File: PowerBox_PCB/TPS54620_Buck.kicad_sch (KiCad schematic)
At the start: 17 parts

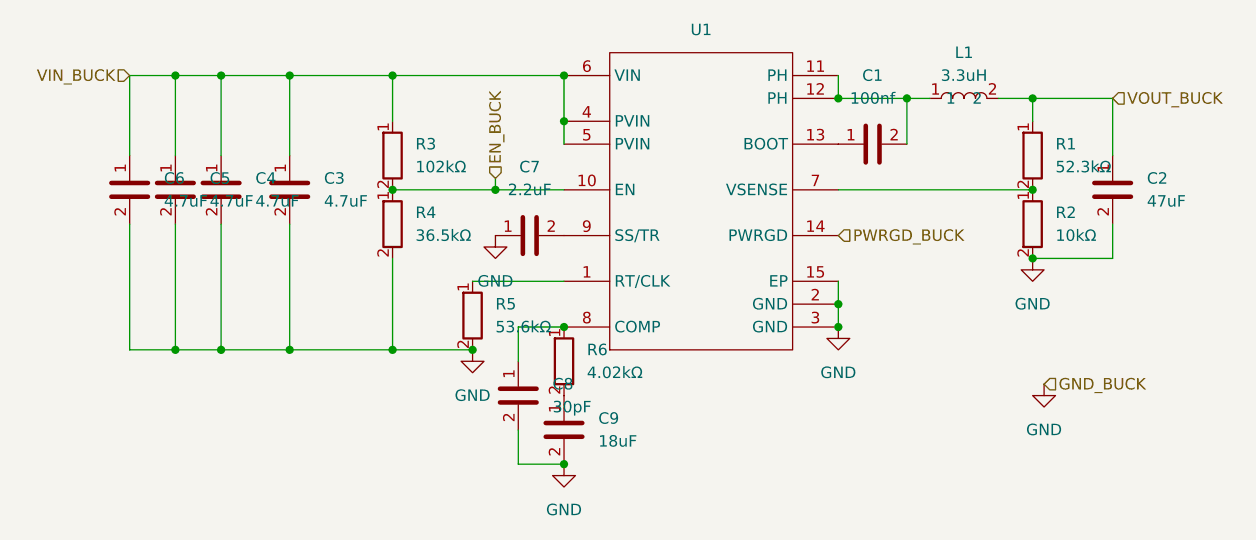
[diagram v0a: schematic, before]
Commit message: .
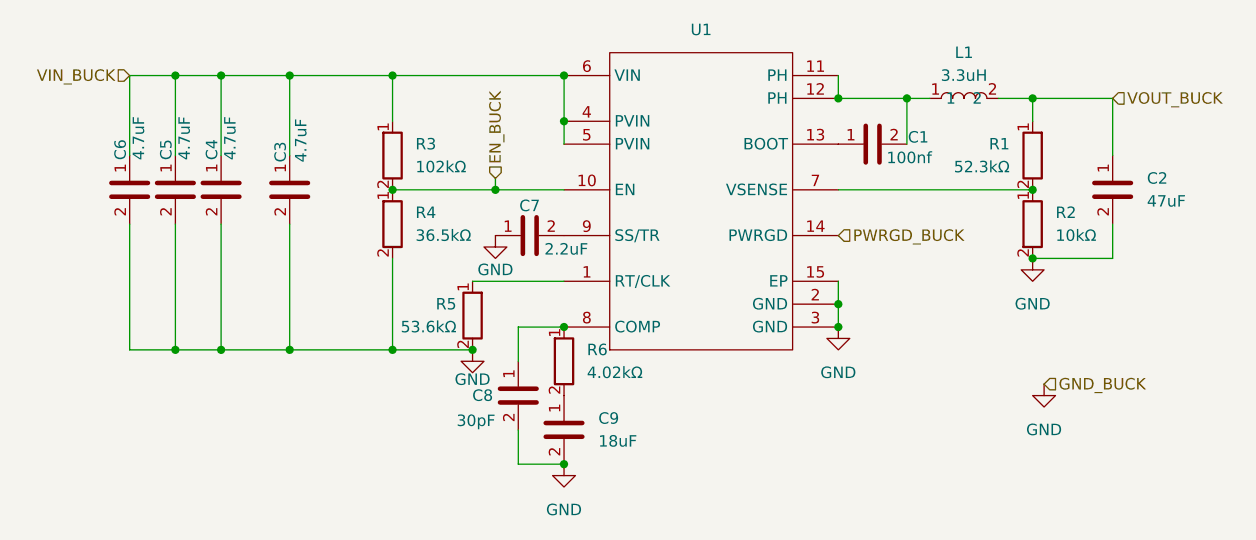
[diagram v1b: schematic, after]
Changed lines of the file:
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@@
 		(lib_id "Buck_TPS54620:30pF_Cap_0805")
 		(at 119.38 115.57 0)
-		(unit 1)
-		(body_style 1)
-		(exclude_from_sim no)
-		(in_bom yes)
-		(on_board yes)
-		(in_pos_files yes)
-		(dnp no)
-		(fields_autoplaced yes)
+		(mirror y)
+		(unit 1)
+		(body_style 1)
+		(exclude_from_sim no)
+		(in_bom yes)
+		(on_board yes)
+		(in_pos_files yes)
+		(dnp no)
 		(property "Reference" "C8"
-			(at 123.19 114.2999 0)
+			(at 116.586 115.57 0)
 			(show_name no)
 			(do_not_autoplace no)
@@
 		)
 		(property "Value" "30pF"
-			(at 123.19 116.8399 0)
+			(at 116.84 118.364 0)
 			(show_name no)
 			(do_not_autoplace no)
@@
 		(lib_id "Buck_TPS54620:53.6kΩ_Res_0805")
 		(at 114.3 106.68 0)
-		(unit 1)
-		(body_style 1)
-		(exclude_from_sim no)
-		(in_bom yes)
-		(on_board yes)
-		(in_pos_files yes)
-		(dnp no)
-		(fields_autoplaced yes)
+		(mirror y)
+		(unit 1)
+		(body_style 1)
+		(exclude_from_sim no)
+		(in_bom yes)
+		(on_board yes)
+		(in_pos_files yes)
+		(dnp no)
 		(property "Reference" "R5"
-			(at 116.84 105.4099 0)
+			(at 112.522 105.41 0)
 			(show_name no)
 			(do_not_autoplace no)
@@
 		)
 		(property "Value" "53.6kΩ"
-			(at 116.84 107.9499 0)
+			(at 112.522 107.95 0)
 			(show_name no)
 			(do_not_autoplace no)
@@
 		(in_pos_files yes)
 		(dnp no)
-		(fields_autoplaced yes)
 		(property "Reference" "C7"
-			(at 120.65 90.17 90)
+			(at 120.65 94.488 90)
 			(show_name no)
 			(do_not_autoplace no)
@@
 		)
 		(property "Value" "2.2uF"
-			(at 120.65 92.71 90)
+			(at 124.714 99.314 90)
 			(show_name no)
 			(do_not_autoplace no)
@@
 		(in_pos_files yes)
 		(dnp no)
-		(fields_autoplaced yes)
 		(property "Reference" "C5"
-			(at 85.09 91.4399 0)
+			(at 80.264 89.408 90)
 			(show_name no)
 			(do_not_autoplace no)
@@
 		)
 		(property "Value" "4.7uF"
-			(at 85.09 93.9799 0)
+			(at 82.296 89.408 90)
 			(show_name no)
 			(do_not_autoplace no)
@@
 		(in_pos_files yes)
 		(dnp no)
-		(fields_autoplaced yes)
 		(property "Reference" "C6"
-			(at 80.01 91.4399 0)
+			(at 75.184 89.408 90)
 			(show_name no)
 			(do_not_autoplace no)
@@
 		)
 		(property "Value" "4.7uF"
-			(at 80.01 93.9799 0)
+			(at 77.216 89.408 90)
 			(show_name no)
 			(do_not_autoplace no)
@@
 		(in_pos_files yes)
 		(dnp no)
-		(fields_autoplaced yes)
 		(property "Reference" "C4"
-			(at 90.17 91.4399 0)
+			(at 85.344 89.408 90)
 			(show_name no)
 			(do_not_autoplace no)
@@
 		)
 		(property "Value" "4.7uF"
-			(at 90.17 93.9799 0)
+			(at 87.376 89.408 90)
 			(show_name no)
 			(do_not_autoplace no)
@@
 		(in_pos_files yes)
 		(dnp no)
-		(fields_autoplaced yes)
 		(property "Reference" "C3"
-			(at 97.79 91.4399 0)
+			(at 92.964 89.662 90)
 			(show_name no)
 			(do_not_autoplace no)
@@
 		)
 		(property "Value" "4.7uF"
-			(at 97.79 93.9799 0)
+			(at 95.25 89.662 90)
 			(show_name no)
 			(do_not_autoplace no)
@@
 		(in_pos_files yes)
 		(dnp no)
-		(fields_autoplaced yes)
 		(property "Reference" "#PWR04"
 			(at 116.84 104.14 0)
@@
 		)
 		(property "Value" "GND"
-			(at 116.84 102.87 0)
+			(at 116.84 101.6 0)
 			(show_name no)
 			(do_not_autoplace no)
@@
 		(in_pos_files yes)
 		(dnp no)
-		(fields_autoplaced yes)
 		(property "Reference" "#PWR03"
 			(at 114.3 116.84 0)
@@
 		)
 		(property "Value" "GND"
-			(at 114.3 115.57 0)
+			(at 114.3 113.792 0)
 			(show_name no)
 			(do_not_autoplace no)
@@
 		(in_pos_files yes)
 		(dnp no)
-		(fields_autoplaced yes)
 		(property "Reference" "C1"
-			(at 158.75 80.01 90)
+			(at 163.83 86.868 90)
 			(show_name no)
 			(do_not_autoplace no)
@@
 		)
 		(property "Value" "100nf"
-			(at 158.75 82.55 90)
+			(at 162.814 89.154 90)
 			(show_name no)
 			(do_not_autoplace no)
@@
 		(lib_id "Buck_TPS54620:52.3kΩ_Res_0805")
 		(at 176.53 88.9 0)
-		(unit 1)
-		(body_style 1)
-		(exclude_from_sim no)
-		(in_bom yes)
-		(on_board yes)
-		(in_pos_files yes)
-		(dnp no)
-		(fields_autoplaced yes)
+		(mirror y)
+		(unit 1)
+		(body_style 1)
+		(exclude_from_sim no)
+		(in_bom yes)
+		(on_board yes)
+		(in_pos_files yes)
+		(dnp no)
 		(property "Reference" "R1"
-			(at 179.07 87.6299 0)
+			(at 173.99 87.6299 0)
 			(show_name no)
 			(do_not_autoplace no)
@@
 		)
 		(property "Value" "52.3kΩ"
-			(at 179.07 90.1699 0)
-			(show_name no)
-			(do_not_autoplace no)
+			(at 173.99 90.1699 0)
+			(show_name no)
+			(do_not_autoplace no)
